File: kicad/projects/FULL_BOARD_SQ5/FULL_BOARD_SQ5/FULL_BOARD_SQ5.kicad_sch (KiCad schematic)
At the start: 52 parts, among them J1 Conn_ARM_JTAG_SWD_10, J2 UART, J3 USB_C_Receptacle_USB2.0_16P, J4 CONN_2x1, Q1 BC847, SW1 TL3342F450QG, U1 24LC512, U3 AP2112K-3.3, U4 AP2112K-3.3, U73 STM32L433CCTx, Y1 NX3215SA-32.768KHZ-EXS00A-MU0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

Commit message: saving work
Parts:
- D2: footprint Package_TO_SOT_SMD_AKL:SOT-23 -> PCM_Package_TO_SOT_SMD_AKL:SOT-23
- D7: footprint Package_SO_AKL:TSOP-6_1.65x3.05mm_P0.95mm -> PCM_Package_SO_AKL:TSOP-6_1.65x3.05mm_P0.95mm
- J3: footprint Connector_USB:USB_C_Receptacle_GCT_USB4105-xx-A_16P_TopMnt_Horizontal_Modified -> Connector_USB:USB_C_Receptacle_GCT_USB4105-xx-A_16P_TopMnt_Horizontal
- Y1: footprint Crystal_AKL:Crystal_SMD_MicroCrystal_CC7V-T1A-2Pin_3.2x1.5mm_HandSoldering -> PCM_Crystal_AKL:Crystal_SMD_MicroCrystal_CC7V-T1A-2Pin_3.2x1.5mm_HandSoldering
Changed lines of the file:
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@@
 			)
 		)
-		(property "Footprint" "Connector_USB:USB_C_Receptacle_GCT_USB4105-xx-A_16P_TopMnt_Horizontal_Modified"
+		(property "Footprint" "Connector_USB:USB_C_Receptacle_GCT_USB4105-xx-A_16P_TopMnt_Horizontal"
 			(at 328.93 184.15 0)
 			(effects
@@
 			)
 		)
-		(property "Footprint" "Crystal_AKL:Crystal_SMD_MicroCrystal_CC7V-T1A-2Pin_3.2x1.5mm_HandSoldering"
+		(property "Footprint" "PCM_Crystal_AKL:Crystal_SMD_MicroCrystal_CC7V-T1A-2Pin_3.2x1.5mm_HandSoldering"
 			(at 133.35 68.58 0)
 			(effects
@@
 			)
 		)
-		(property "Footprint" "Package_SO_AKL:TSOP-6_1.65x3.05mm_P0.95mm"
+		(property "Footprint" "PCM_Package_SO_AKL:TSOP-6_1.65x3.05mm_P0.95mm"
 			(at 370.84 198.12 0)
 			(effects
@@
 			)
 		)
-		(property "Footprint" "Package_TO_SOT_SMD_AKL:SOT-23"
+		(property "Footprint" "PCM_Package_TO_SOT_SMD_AKL:SOT-23"
 			(at 328.93 31.75 0)
 			(effects

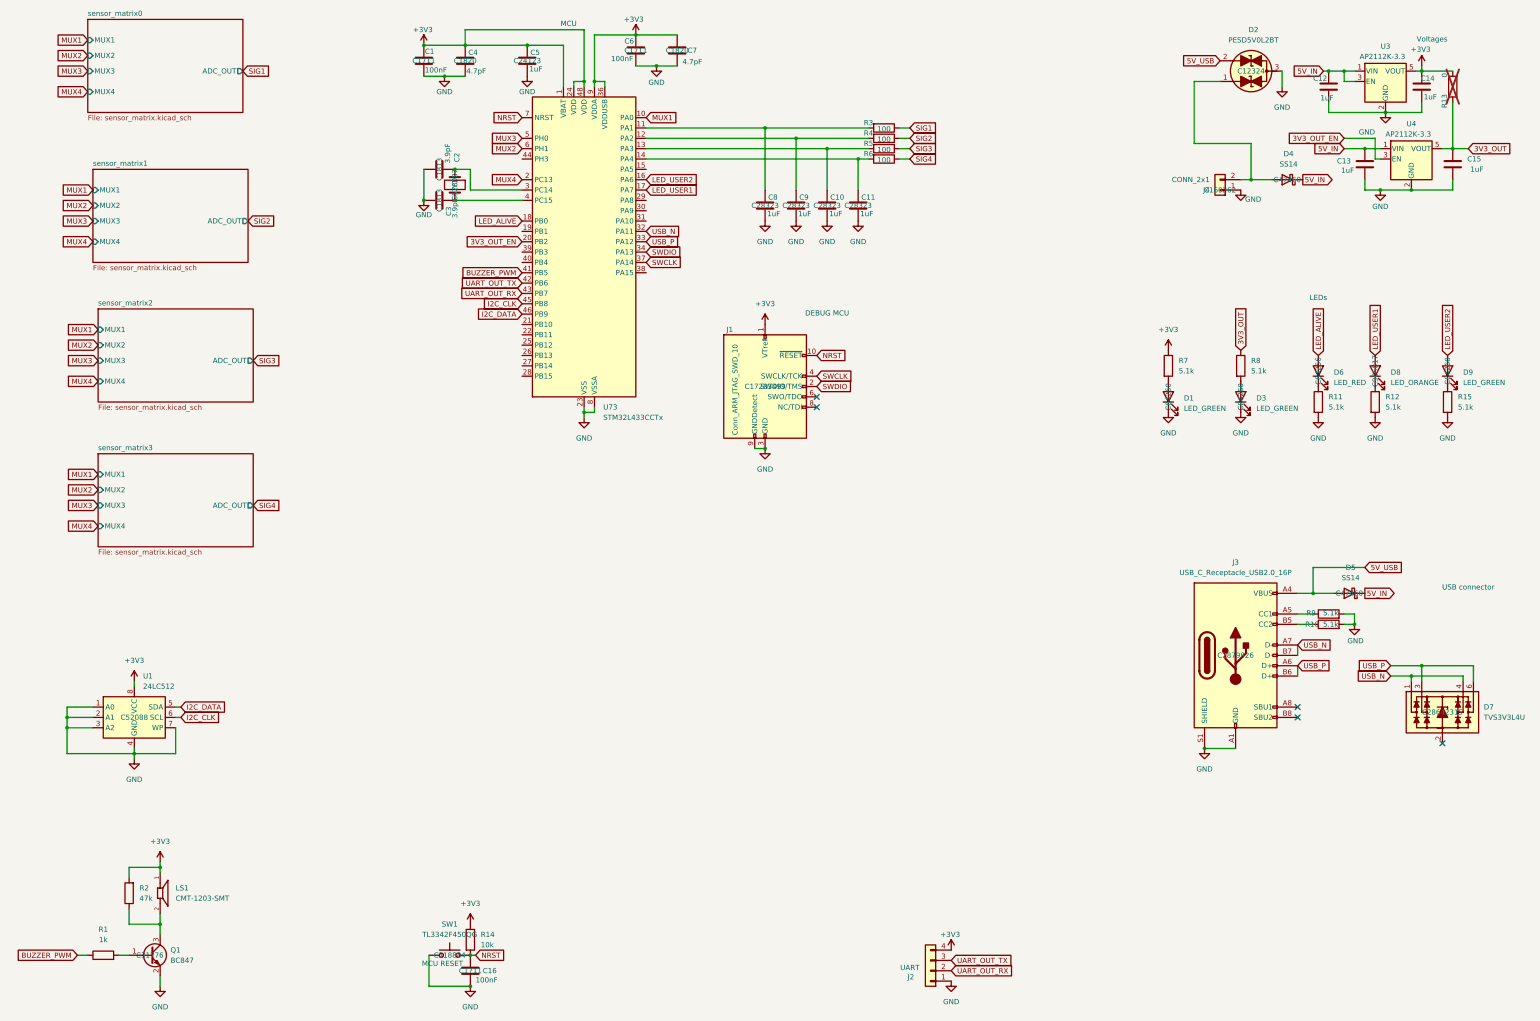
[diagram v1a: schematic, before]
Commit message: all sensors placed and first connections
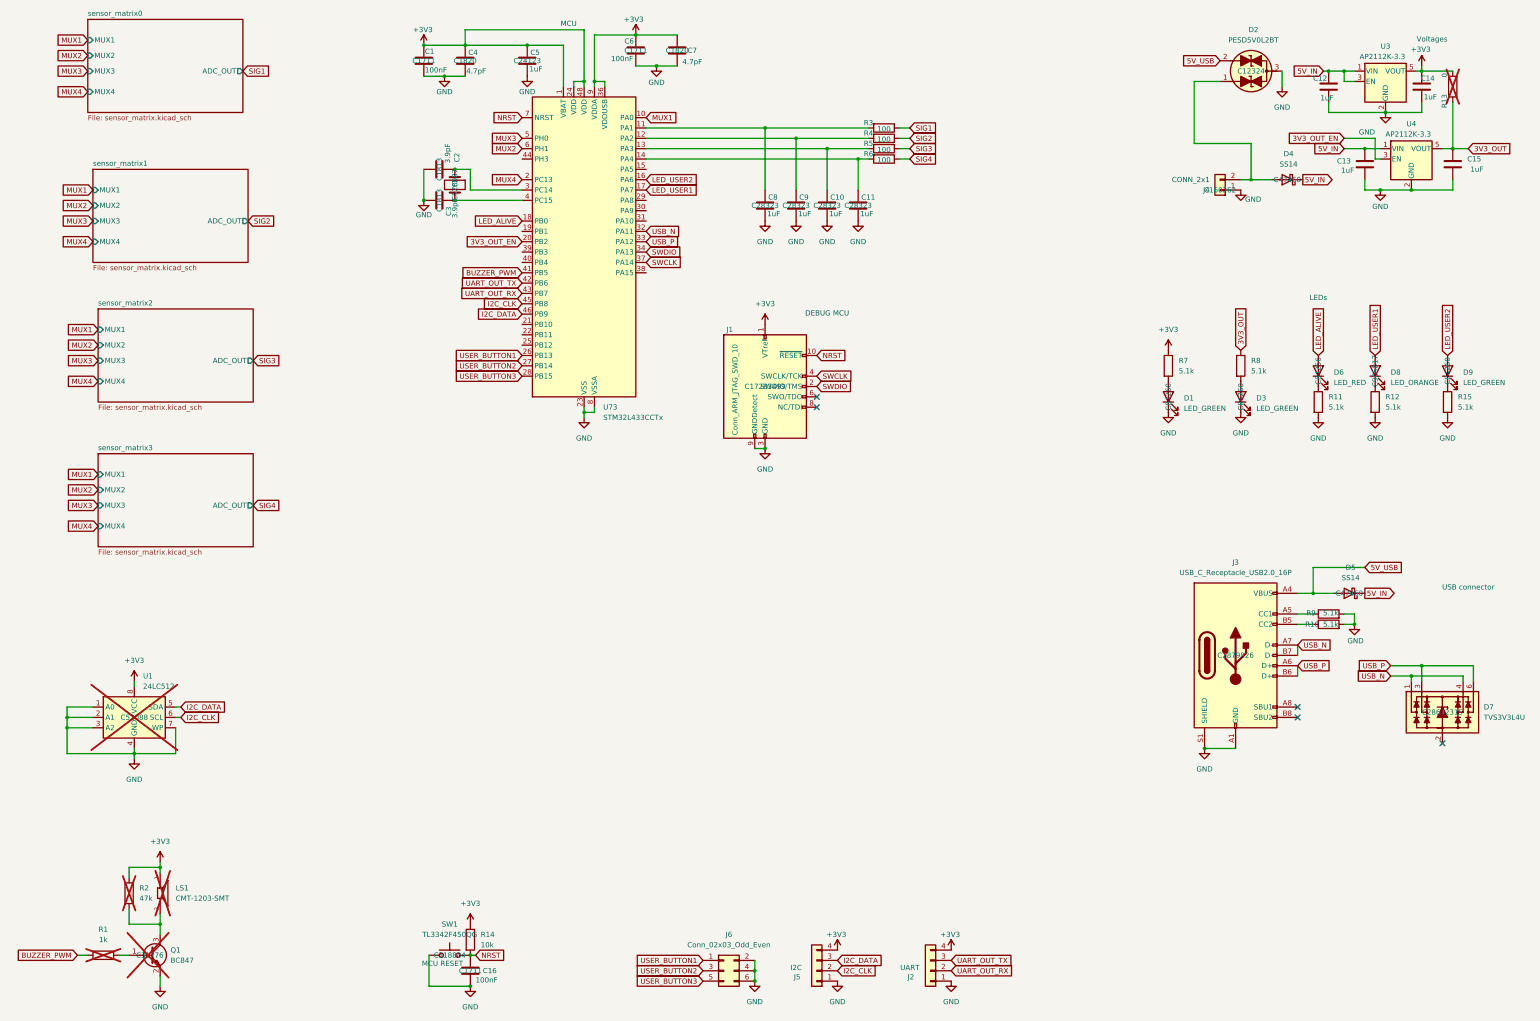
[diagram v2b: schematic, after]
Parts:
- added J5: I2C, Connector_PinHeader_2.54mm:PinHeader_1x04_P2.54mm_Vertical, symbol Connector_Generic:Conn_01x04
- added J6: Conn_02x03_Odd_Even, Connector_PinHeader_2.54mm:PinHeader_2x03_P2.54mm_Vertical, symbol Connector_Generic:Conn_02x03_Odd_Even
- LS1, Q1, R1, R2, U1: now not fitted
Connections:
- net +3V3: now also J5.4 (Pin_4)
- net GND: now also J5.1 (Pin_1), J6.2 (Pin_2), J6.4 (Pin_4), J6.6 (Pin_6)
- net I2C_CLK: now also J5.2 (Pin_2)
- net I2C_DATA: now also J5.3 (Pin_3)
- net USER_BUTTON1: now reaches U73.26 (PB13)
- net USER_BUTTON1: now also J6.1 (Pin_1)
- net USER_BUTTON2: now reaches U73.27 (PB14)
- net USER_BUTTON2: now also J6.3 (Pin_3)
- net USER_BUTTON3: now reaches U73.28 (PB15)
- net USER_BUTTON3: now also J6.5 (Pin_5)

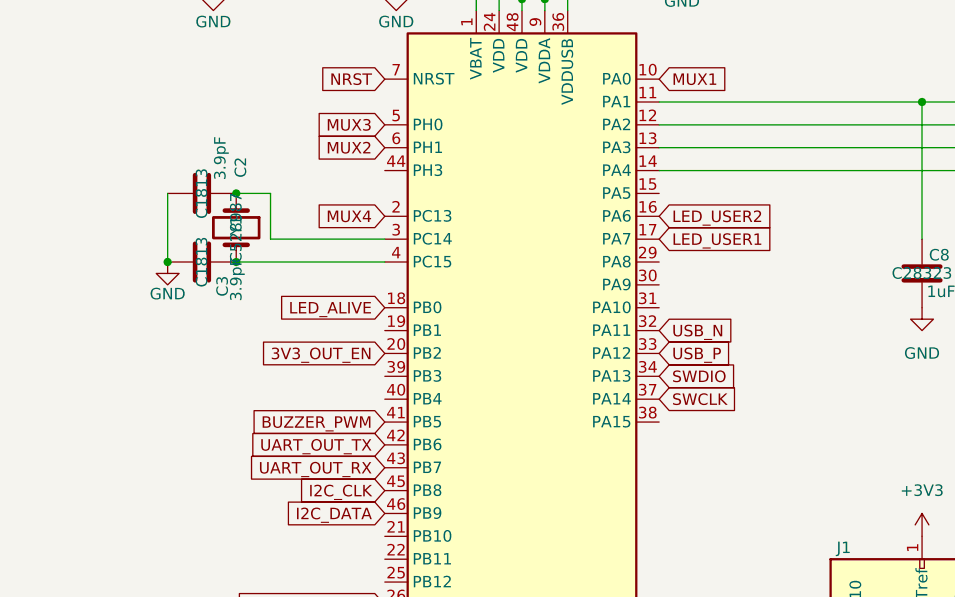
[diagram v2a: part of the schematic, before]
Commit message: some configs
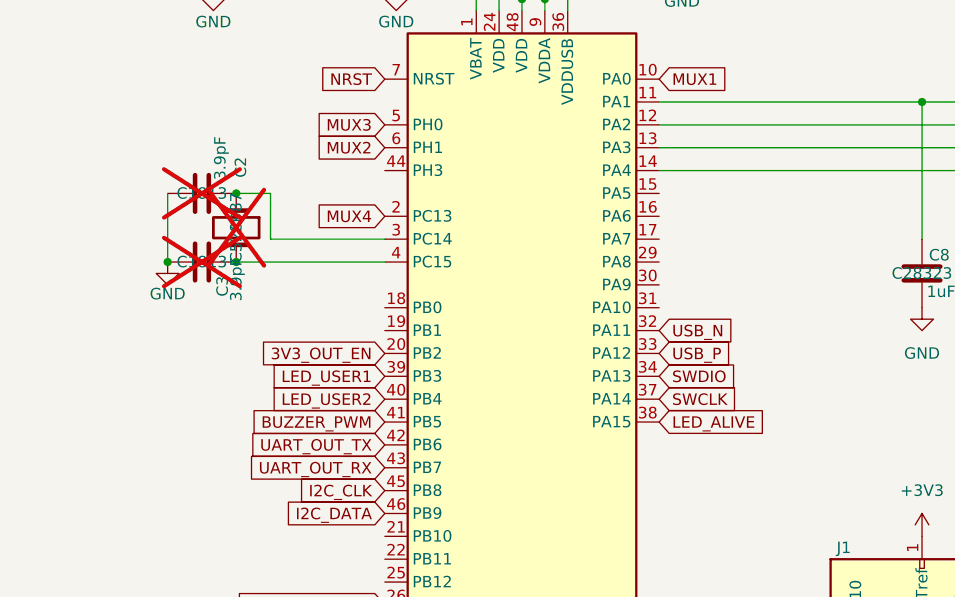
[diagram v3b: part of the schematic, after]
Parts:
- C2, C3, Y1: now not fitted
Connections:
- net LED_ALIVE: now also U73.38 (PA15); no longer U73.18 (PB0)
- net LED_USER1: now also U73.39 (PB3); no longer U73.17 (PA7)
- net LED_USER2: now also U73.40 (PB4); no longer U73.16 (PA6)
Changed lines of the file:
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@@
 		)
 	)
-	(global_label "LED_USER2"
+	(global_label "LED_USER1"
 		(shape input)
-		(at 180.34 67.31 0)
+		(at 149.86 85.09 180)
 		(fields_autoplaced yes)
 		(effects
@@
 				(size 1.27 1.27)
 			)
-			(justify left)
+			(justify right)
 		)
 		(property "Intersheetrefs" "${INTERSHEET_REFS}"
-			(at 193.9084 67.31 0)
+			(at 136.2916 85.09 0)
 			(effects
 				(font
 					(size 1.27 1.27)
 				)
-				(justify left)
+				(justify right)
 				(hide yes)
 			)
@@
 		)
 	)
-	(global_label "LED_ALIVE"
-		(shape input)
-		(at 149.86 77.47 180)
-		(fields_autoplaced yes)
-		(effects
-			(font
-				(size 1.27 1.27)
-			)
-			(justify right)
-		)
-		(property "Intersheetrefs" "${INTERSHEET_REFS}"
-			(at 137.501 77.47 0)
-			(effects
-				(font
-					(size 1.27 1.27)
-				)
-				(justify right)
-				(hide yes)
-			)
-		)
-	)
 	(global_label "I2C_CLK"
 		(shape input)
@@
 		)
 	)
-	(global_label "LED_USER1"
-		(shape input)
-		(at 180.34 69.85 0)
-		(fields_autoplaced yes)
-		(effects
-			(font
-				(size 1.27 1.27)
-			)
-			(justify left)
-		)
-		(property "Intersheetrefs" "${INTERSHEET_REFS}"
-			(at 193.9084 69.85 0)
-			(effects
-				(font
-					(size 1.27 1.27)
-				)
-				(justify left)
-				(hide yes)
-			)
-		)
-	)
 	(global_label "MUX3"
 		(shape input)
@@
 		)
 	)
+	(global_label "LED_USER2"
+		(shape input)
+		(at 149.86 87.63 180)
+		(fields_autoplaced yes)
+		(effects
+			(font
+				(size 1.27 1.27)
+			)
+			(justify right)
+		)
+		(property "Intersheetrefs" "${INTERSHEET_REFS}"
+			(at 136.2916 87.63 0)
+			(effects
+				(font
+					(size 1.27 1.27)
+				)
+				(justify right)
+				(hide yes)
+			)
+		)
+	)
+	(global_label "LED_ALIVE"
+		(shape input)
+		(at 180.34 90.17 0)
+		(fields_autoplaced yes)
+		(effects
+			(font
+				(size 1.27 1.27)
+			)
+			(justify left)
+		)
+		(property "Intersheetrefs" "${INTERSHEET_REFS}"
+			(at 192.699 90.17 0)
+			(effects
+				(font
+					(size 1.27 1.27)
+				)
+				(justify left)
+				(hide yes)
+			)
+		)
+	)
 	(global_label "I2C_CLK"
 		(shape input)
@@
 		(in_bom yes)
 		(on_board yes)
-		(dnp no)
+		(dnp yes)
 		(property "Reference" "C3"
 			(at 131.826 73.914 0)
@@
 		)
 		(property "LCSC p/n" "C1813"
-			(at 129.54 72.39 0)
+			(at 129.54 72.39 90)
 			(effects
 				(font
@@
 		(in_bom yes)
 		(on_board yes)
-		(dnp no)
+		(dnp yes)
 		(property "Reference" "Y1"
 			(at 133.35 68.326 0)
@@
 		(in_bom yes)
 		(on_board yes)
-		(dnp no)
+		(dnp yes)
 		(property "Reference" "C2"
 			(at 133.858 60.706 0)
@@
 		)
 		(property "LCSC p/n" "C1813"
-			(at 129.54 64.77 0)
+			(at 129.54 64.77 90)
 			(effects
 				(font
